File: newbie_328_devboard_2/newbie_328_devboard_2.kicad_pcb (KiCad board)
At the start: 2 copper layers, 100 x 100 mm, 43 parts, among them J1 Conn_02x03_Odd_Even, J2 Conn_01x04, J3 Conn_01x04, J4 Conn_01x04, J5 Conn_02x03_Odd_Even, J6 Conn_01x02, J7 Conn_01x02, SW1 SW_Push, U1 ATmega328-A, U2 LM2576S-5, U3 MCP2515-xST, U4 TJA1050T_CM_118, Y1 20MHz, Y2 Crystal

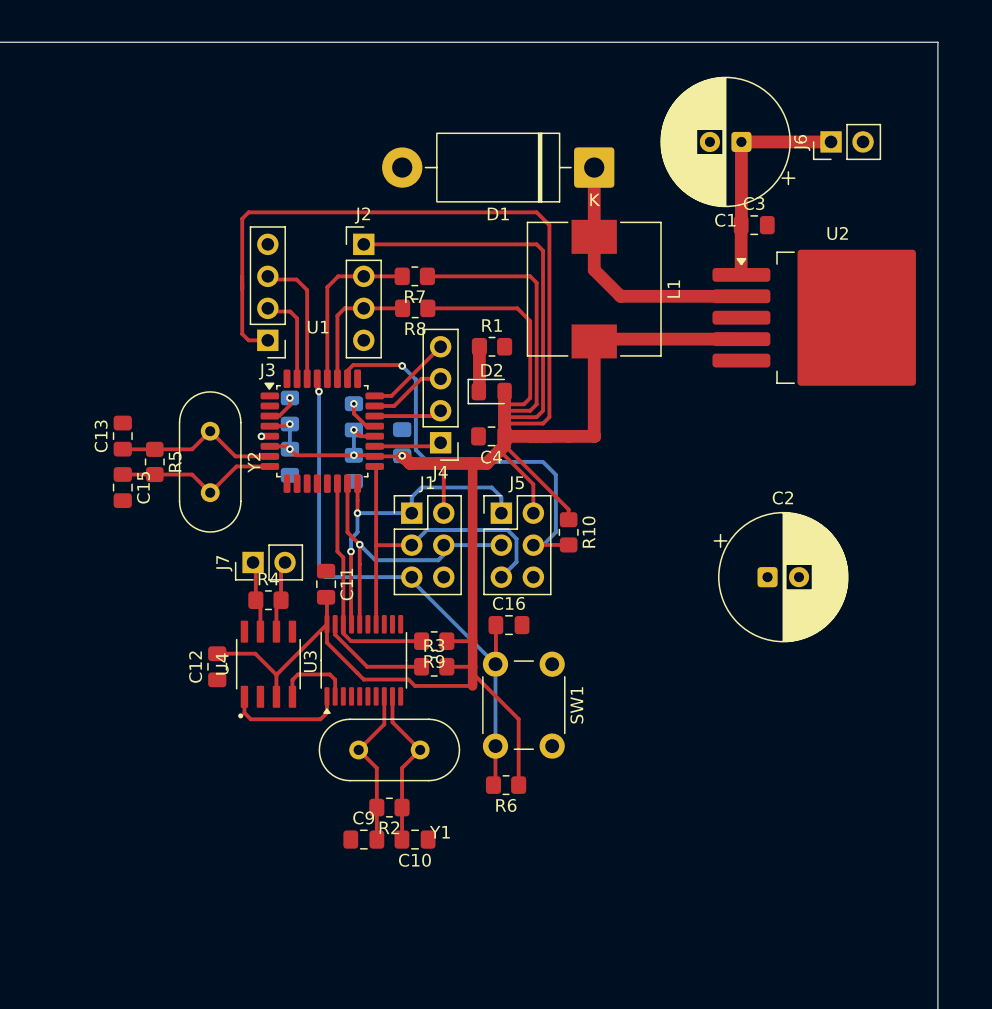
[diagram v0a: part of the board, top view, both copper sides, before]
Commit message: Second iteration of PCB
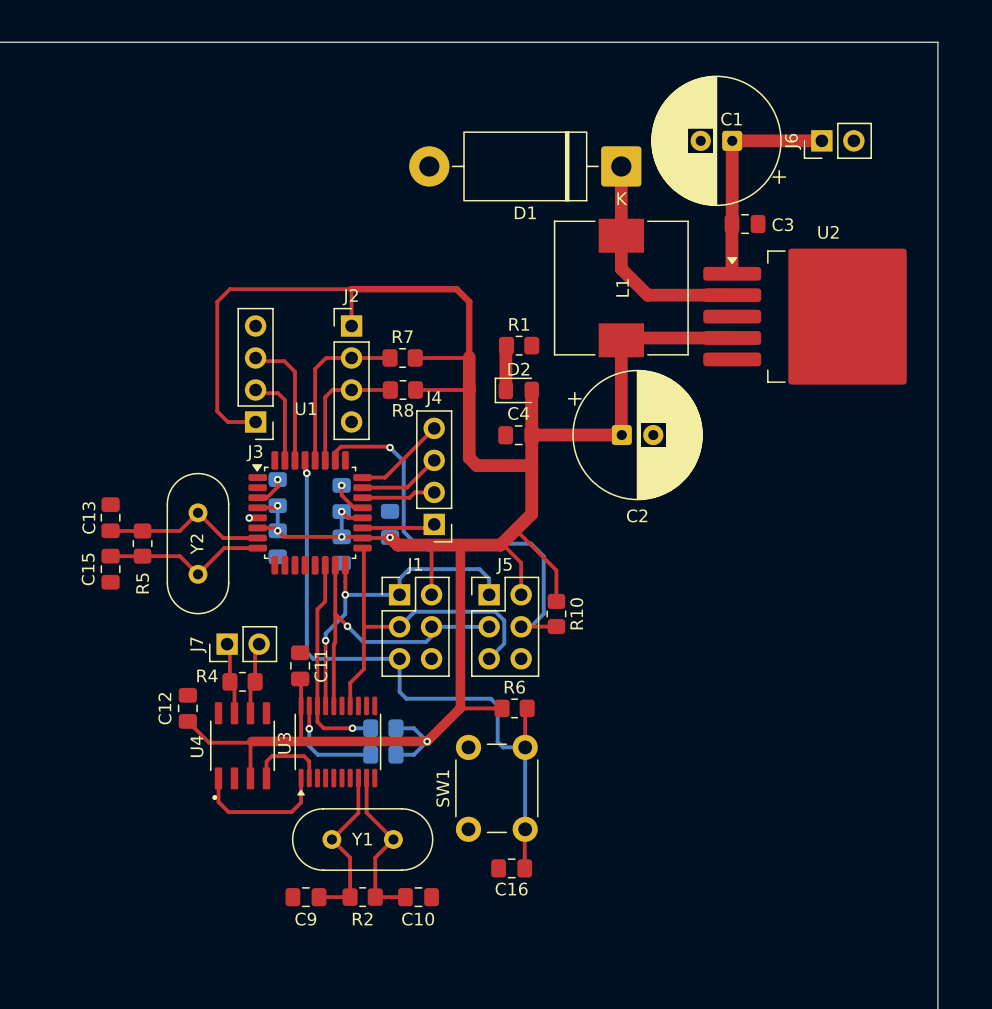
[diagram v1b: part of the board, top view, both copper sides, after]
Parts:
- R3, R9: moved to B.Cu
- moved C16 19.3 mm to (166.2, 115.6), turned to 180 degrees
- moved C2 16.2 mm to (174.9, 81.2)
- moved SW1 14.7 mm to (162.7, 112.5), turned to 90 degrees
- moved R3 8.07 mm to (156.0, 106.5)
- moved R9 8.01 mm to (156.0, 104.5)
- moved R2 7.42 mm to (154.3, 117.9)
- moved Y1 7.42 mm to (156.8, 113.3)
- moved C11 6.80 mm to (149.4, 99.5)
- moved J7 6.80 mm to (143.6, 97.8)
- moved R4 6.80 mm to (144.8, 100.8)
- moved U3 6.80 mm to (152.4, 105.5)
- moved U4 6.80 mm to (144.8, 105.8)
- moved C13 6.55 mm to (134.3, 87.7)
- moved C15 6.55 mm to (134.3, 91.8)
- moved C6 6.55 mm to (152.7, 90.3)
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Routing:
- net +5V: track 263.9 -> 199.7 mm, vias 5 -> 6
- net /RST: track 45.3 -> 51.8 mm
- net Net-(D1-K): track 20.7 -> 17.8 mm
- net /CAN_TX: track 9.56 -> 11.0 mm
- net /SS: track 18.6 -> 17.1 mm, vias 0 -> 1
- net /MOSI: track 25.0 -> 26.1 mm
- net Net-(U3-OSC2): track 12.8 -> 13.4 mm
- net Net-(U3-~{RESET}): track 8.75 -> 8.36 mm, vias 0 -> 1
